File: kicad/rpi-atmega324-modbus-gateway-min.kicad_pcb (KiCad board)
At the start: 2 copper layers, 68 x 64.4 mm, 73 parts, among them J1 Raspberry_Pi_2+, J10 Conn_01x02, J11 Conn_01x02, J12 Conn_01x02, J13 Conn_01x02, J14 Screw_Terminal_01x02, J15 Screw_Terminal_01x02, J16 Conn_01x11, J17 Conn_01x11, J18 Conn_01x11, J19 Conn_01x11, J2 UART-Harwin3, J3 Conn_01x02, J4 Conn_02x03_Odd_Even, J5 Atmega-ISP-6, J6 Conn_01x03, J7 Conn_01x03, J8 Conn_01x02, J9 Conn_01x02, SW1 SW_Push, SW2 SW_SPST, U1 ATMEGA324P-20AU, U2 SN65HVD11, U3 SN65HVD11, Y1 12MHz

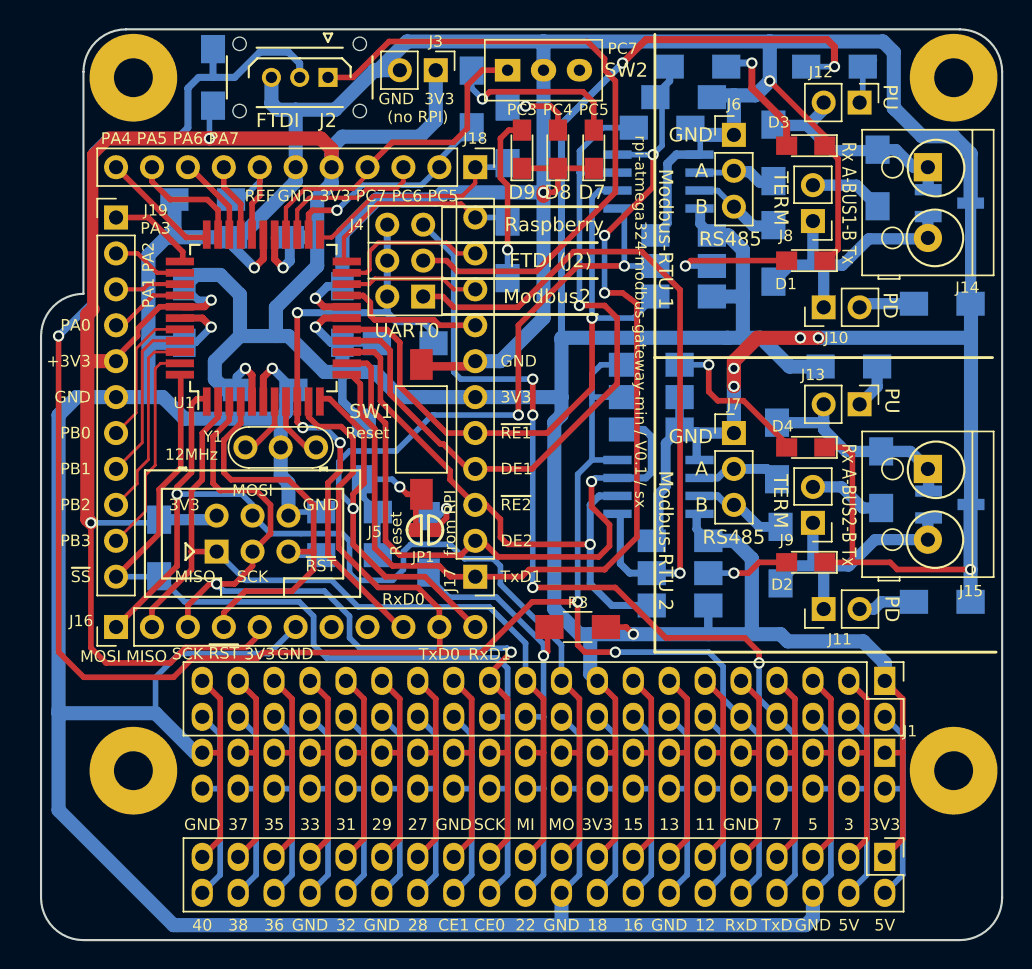
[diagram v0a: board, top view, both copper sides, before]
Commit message: V0.2 Tapeout
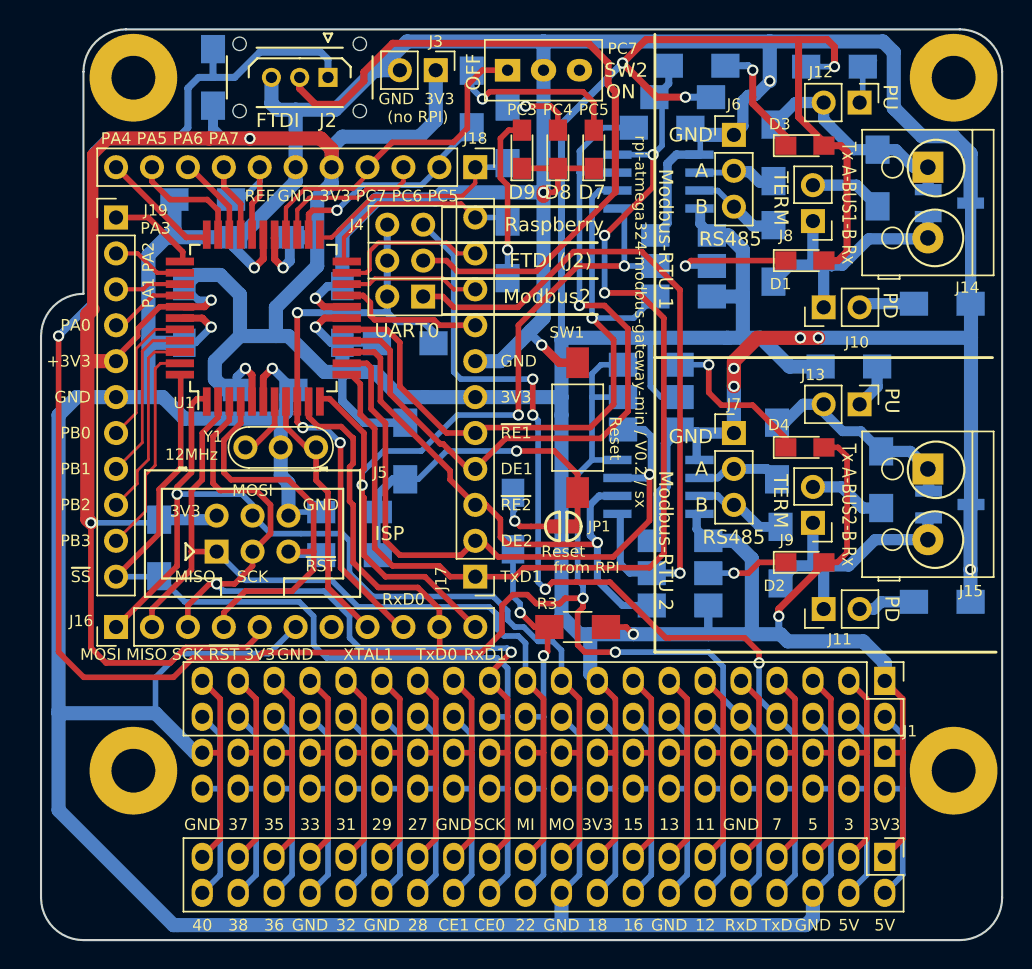
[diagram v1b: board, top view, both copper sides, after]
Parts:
- C2: value 100n -> 1n
- moved SW1 11.0 mm to (156.1, 78.6)
- moved JP1 9.78 mm to (155.1, 85.6), turned to 0 degrees
- moved C1 6.19 mm to (151.5, 85.2)
- moved R1 2.92 mm to (143.9, 80.3)
- moved R9 0.09 mm to (164.5, 53.0), turned to 0 degrees
- moved R14 0.06 mm to (163.5, 55.2), turned to 0 degrees
- moved D1 0.06 mm to (172.1, 66.8), turned to 0 degrees
- moved D2 0.06 mm to (172.1, 88.1), turned to 0 degrees
- moved D3 0.06 mm to (172.1, 58.7), turned to 0 degrees
- moved D4 0.06 mm to (172.1, 80.0), turned to 0 degrees
- turned R10 to 0 degrees
- turned R16 to 0 degrees
- turned R7 to 0 degrees
- turned R8 to 0 degrees
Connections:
- D1 pad 1: GND -> Net-(D1-Pad1)
- D1 pad 2: Net-(D1-Pad2) -> +3V3
- D2 pad 1: GND -> Net-(D2-Pad1)
- D2 pad 2: Net-(D2-Pad2) -> +3V3
- D3 pad 1: GND -> Net-(D3-Pad1)
- D3 pad 2: Net-(D3-Pad2) -> +3V3
- D4 pad 1: GND -> Net-(D4-Pad1)
- D4 pad 2: Net-(D4-Pad2) -> +3V3
- J16 pad 8: Net-(J16-Pad8) -> /XTAL1
- J2 pad 1: Net-(J2-Pad1) -> /TxD0
- J2 pad 2: /TxD0 -> Net-(J2-Pad2)
- J4 pad 3: Net-(J2-Pad1) -> Net-(J2-Pad2)
- R10 pad 1: Net-(D4-Pad2) -> /TxD0
- R10 pad 2: /TxD0 -> Net-(D4-Pad1)
- R14 pad 1: GND -> /TxD1
- R14 pad 2: /TxD1 -> +3V3
- R16 pad 1: GND -> /TxD0
- R16 pad 2: /TxD0 -> +3V3
- R7 pad 1: Net-(D1-Pad2) -> /RxD1
- R7 pad 2: /RxD1 -> Net-(D1-Pad1)
- R8 pad 1: Net-(D2-Pad2) -> /Modbus/TxD2
- R8 pad 2: /Modbus/TxD2 -> Net-(D2-Pad1)
- R9 pad 1: Net-(D3-Pad2) -> /TxD1
- R9 pad 2: /TxD1 -> Net-(D3-Pad1)
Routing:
- net +3V3: track 351.5 -> 405.7 mm, vias 9 -> 11
- net Net-(J2-Pad2): track 0.00 -> 51.4 mm
- net Net-(J2-Pad1): track 47.1 -> 0.00 mm
- net GND: track 491.4 -> 453.2 mm, vias 11 -> 12
- net /XTAL1: track 4.63 -> 18.8 mm
- net Net-(C2-Pad1): track 12.5 -> 24.2 mm
- net Net-(D4-Pad1): track 0.00 -> 11.5 mm, vias 0 -> 1
- net Net-(D4-Pad2): track 11.4 -> 0.00 mm, vias 1 -> 0
- net Net-(D1-Pad2): track 9.19 -> 0.00 mm, vias 1 -> 0
- net Net-(D1-Pad1): track 0.00 -> 9.19 mm, vias 0 -> 1
- net Net-(D3-Pad2): track 8.75 -> 0.00 mm, vias 1 -> 0
- net Net-(D3-Pad1): track 0.00 -> 8.37 mm, vias 0 -> 1
- net Net-(D2-Pad2): track 5.86 -> 0.00 mm, vias 1 -> 0
- net Net-(D2-Pad1): track 0.00 -> 5.79 mm, vias 0 -> 1
- net /RxD1: track 63.0 -> 58.4 mm
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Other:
- board text added: "ISP"
- board text added: "OFF"
- board text added: "ON"
- board text added: "Tx A-BUS1-B Rx"
- board text added: "Tx A-BUS2-B Rx"
- board text added: "XTAL1"
- board text added: "rpi-atmega324-modbus-gateway-min / V0.2 / sx"
- board text removed: "Rx A-BUS1-B Tx"
- board text removed: "Rx A-BUS2-B Tx"
- board text removed: "rpi-atmega324-modbus-gateway-min / V0.1 / sx"
